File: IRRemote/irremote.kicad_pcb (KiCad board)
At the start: 2 copper layers, 22 parts, among them P1 USB_OTG, P2 TL1838_PINHEADER, P3 DS18B20_PINHEADER_TO92, Q1 Q_NPN_BEC (MMBT2222ALT1G, 145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, Q2 Q_NPN_BEC (MMBT2222ALT1G, 145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, Q3 Q_NPN_BEC (MMBT2222ALT1G, 145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, Q4 Q_NPN_BEC (MMBT2222ALT1G, 145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, U1 ESP-12E, U2 AP1117

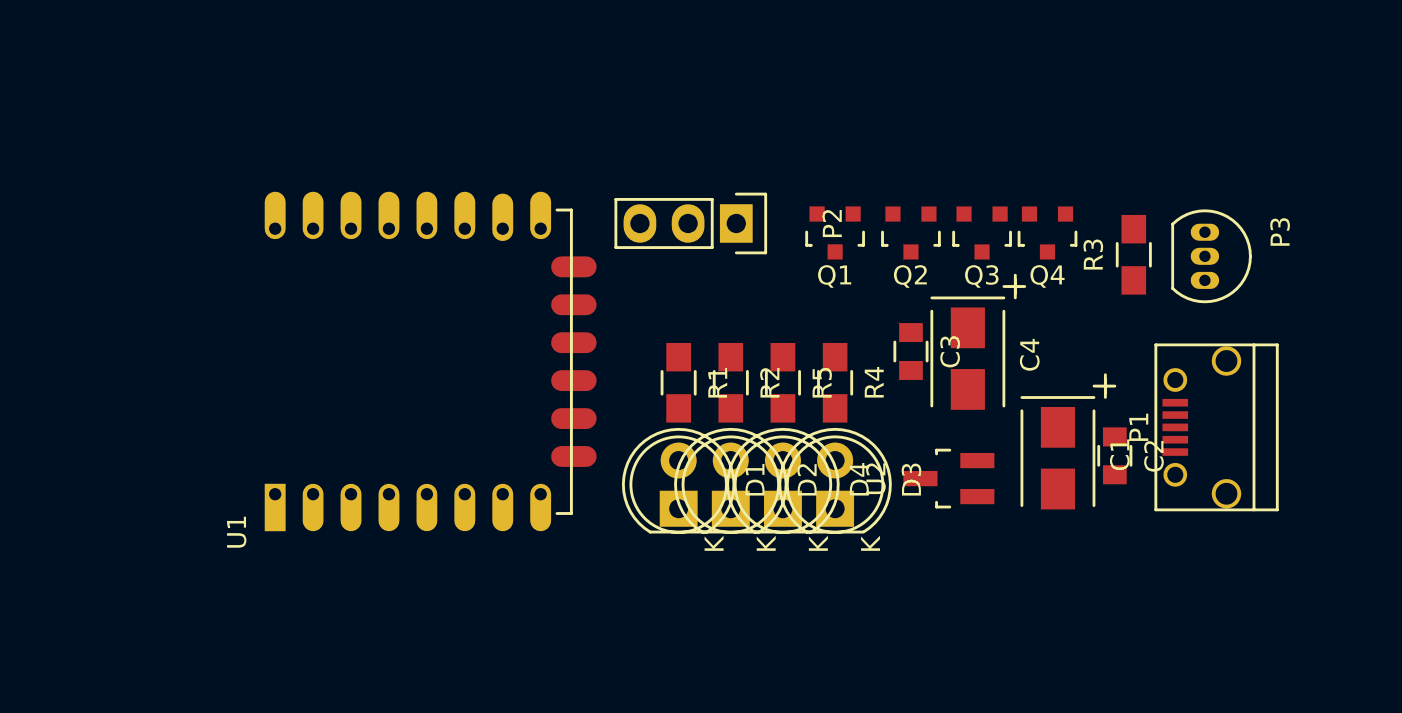
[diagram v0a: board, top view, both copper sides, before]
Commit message: board layout complete
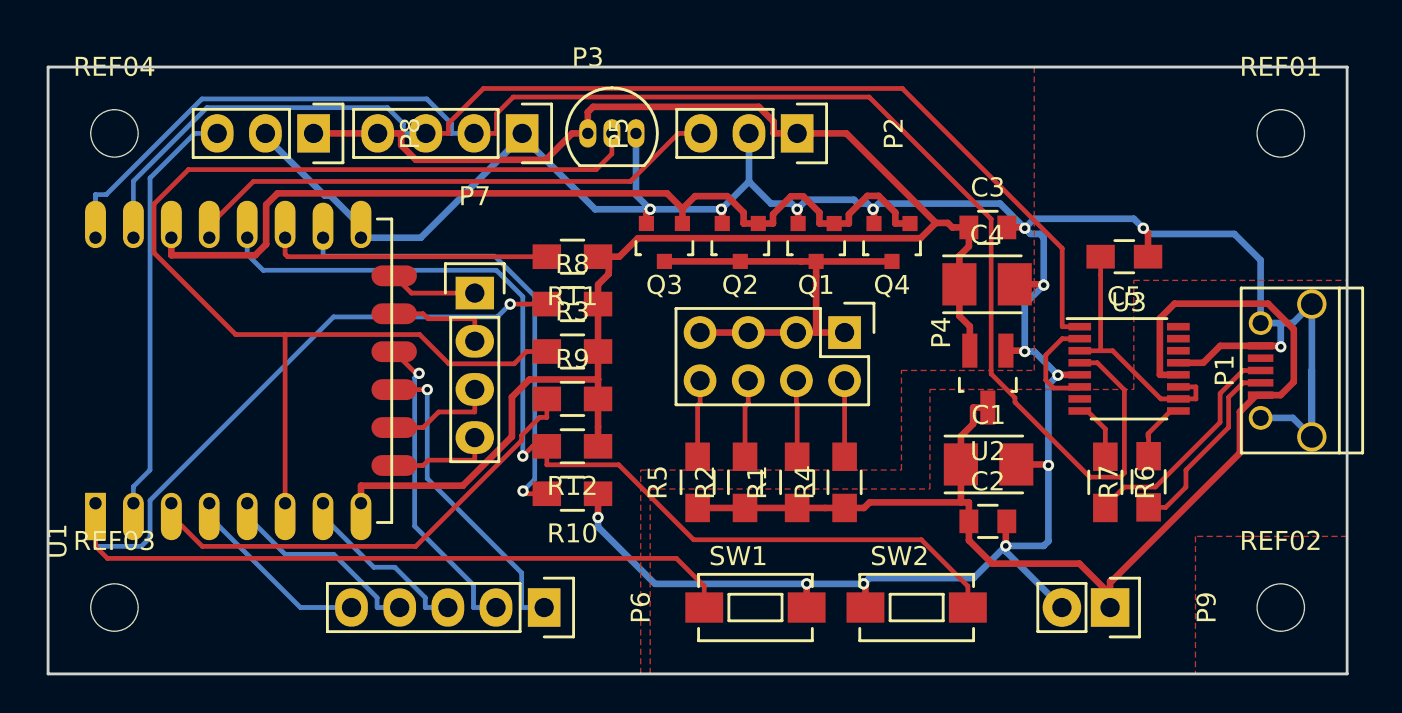
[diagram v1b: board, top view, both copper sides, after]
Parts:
- removed D1, D2, D3, D4: LED, LEDs:LED-5MM
- added C5: C, Capacitors_SMD:C_0805_HandSoldering, F.Cu at (163.2, 61.5)
- added P4: CONN_02X04, Pin_Headers:Pin_Header_Straight_2x04, F.Cu at (148.5, 65.5)
- added P5: CONN_01X04, Pin_Headers:Pin_Header_Straight_1x04, F.Cu at (131.5, 55.0)
- added P6: CONN_01X05, Pin_Headers:Pin_Header_Straight_1x05, F.Cu at (132.7, 80.0)
- added P7: CONN_01X04, Pin_Headers:Pin_Header_Straight_1x04, F.Cu at (129.0, 63.4)
- added P8: TEMP6000, Pin_Headers:Pin_Header_Straight_1x03, F.Cu at (120.5, 55.0)
- added P9: CONN_01X02, Pin_Headers:Pin_Header_Straight_1x02, F.Cu at (162.5, 80.0)
- added R10: 4.7k, Resistors_SMD:R_0805_HandSoldering, F.Cu at (134.2, 74.0)
- added R11: 4.7k, Resistors_SMD:R_0805_HandSoldering, F.Cu at (134.2, 61.5)
- added R12: 4.7k, Resistors_SMD:R_0805_HandSoldering, F.Cu at (134.2, 71.5)
- added R6: 27, Resistors_SMD:R_0805_HandSoldering, F.Cu at (162.2, 73.4)
- added R7: 27, Resistors_SMD:R_0805_HandSoldering, F.Cu at (164.5, 73.4)
- added R8: 4.7k, Resistors_SMD:R_0805_HandSoldering, F.Cu at (134.2, 64.0)
- added R9: 4.7k, Resistors_SMD:R_0805_HandSoldering, F.Cu at (134.2, 69.0)
- added REF01: MountingHole_2-5mm, Mounting_Holes:MountingHole_2-5mm, F.Cu at (171.5, 55.0)
- added REF02: MountingHole_2-5mm, Mounting_Holes:MountingHole_2-5mm, F.Cu at (171.5, 80.0)
- added REF03: MountingHole_2-5mm, Mounting_Holes:MountingHole_2-5mm, F.Cu at (110.0, 80.0)
- added REF04: MountingHole_2-5mm, Mounting_Holes:MountingHole_2-5mm, F.Cu at (110.0, 55.0)
- added SW1: SW_PUSH, Buttons_Switches_SMD:SW_SPST_EVQPE1, F.Cu at (143.8, 80.0)
- added SW2: SW_PUSH, Buttons_Switches_SMD:SW_SPST_EVQPE1, F.Cu at (152.3, 80.0)
- added U3: FT230XS, Housings_SSOP:SSOP-16_3.9x4.9mm_Pitch0.635mm, F.Cu at (163.5, 67.4)
- C1, C4: footprint Capacitors_Tantalum_SMD:TantalC_SizeB_EIA-3528_Wave -> Capacitors_Tantalum_SMD:TantalC_SizeB_EIA-3528_Reflow
- moved P3 33.0 mm to (135.0, 55.0), turned to 0 degrees
- moved R3 30.0 mm to (134.2, 66.5), turned to 0 degrees
- moved Q3 16.8 mm to (139.0, 60.8)
- moved U1 9.49 mm to (109.0, 74.5)
- moved Q2 9.01 mm to (143.0, 60.8)
- moved Q4 8.22 mm to (151.0, 60.8)
- moved R1 8.16 mm to (146.0, 73.4), turned to 90 degrees
- moved C3 7.70 mm to (156.1, 60.0), turned to 0 degrees
- moved C2 7.54 mm to (156.1, 75.5), turned to 0 degrees
- moved R5 6.91 mm to (140.8, 73.4), turned to 90 degrees
- moved P2 5.73 mm to (146.0, 55.0)
- moved U2 5.63 mm to (156.1, 68.0), turned to 180 degrees
- moved P1 5.41 mm to (172.0, 67.5)
- moved R2 5.30 mm to (143.2, 73.4), turned to 90 degrees
- moved R4 5.27 mm to (148.5, 73.4), turned to 90 degrees
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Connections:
- net Net-(D1-Pad1) renamed LED_DR_5
- P1 pad 2: (no net) -> USBDM_1_N
- P1 pad 3: (no net) -> USBDP_1_P
- U1 pad 1: (no net) -> Net-(R8-Pad1)
- U1 pad 10: (no net) -> Net-(P7-Pad3)
- U1 pad 11: (no net) -> Net-(P6-Pad1)
- U1 pad 12: (no net) -> Net-(P6-Pad2)
- U1 pad 13: (no net) -> Net-(P7-Pad2)
- U1 pad 14: (no net) -> Net-(P7-Pad1)
- U1 pad 16: (no net) -> Net-(R10-Pad2)
- U1 pad 17: (no net) -> Net-(R11-Pad2)
- U1 pad 18: (no net) -> Net-(R12-Pad2)
- U1 pad 2: (no net) -> TEMT
- U1 pad 21: (no net) -> TXD_UA_1
- U1 pad 22: (no net) -> RXD_UA_1
- U1 pad 3: (no net) -> Net-(R9-Pad1)
- U1 pad 4: (no net) -> Net-(P6-Pad5)
- U1 pad 5: (no net) -> Net-(P6-Pad4)
- U1 pad 7: (no net) -> Net-(P6-Pad3)
- U1 pad 9: (no net) -> Net-(P7-Pad4)
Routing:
- net GND: track 0.00 -> 163.2 mm, vias 0 -> 15
- net +3V3: track 0.00 -> 93.0 mm
- net RXD_UA_1: track 0.00 -> 81.7 mm
- net Net-(R8-Pad1): track 0.00 -> 68.9 mm, vias 0 -> 1
- net TXD_UA_1: track 0.00 -> 64.3 mm
- net +5V: track 0.00 -> 62.5 mm
- net TEMP_READ: track 0.00 -> 61.2 mm
- net Net-(R12-Pad2): track 0.00 -> 53.2 mm, vias 0 -> 1
- net LED_DR: track 0.00 -> 48.4 mm
- net IR_IN: track 0.00 -> 28.6 mm
- net Net-(R9-Pad1): track 0.00 -> 25.1 mm
- net Net-(R10-Pad2): track 0.00 -> 24.9 mm, vias 0 -> 1
- net LED_DR_5: track 0.00 -> 23.4 mm
- net TEMT: track 0.00 -> 22.0 mm
- net Net-(P6-Pad2): track 0.00 -> 16.7 mm, vias 0 -> 1
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- added copper zone on F.Cu, net +3V3
- added copper zone on F.Cu, net +5V
- added copper zone on B.Cu, net GND
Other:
- board outline added: 68.5 x 32 mm
- net class 3v added: clearance 0.2, trace_width 0.35, via_dia 0.6, via_drill 0.4
- net class 5v added: clearance 0.2, trace_width 0.35, via_dia 0.6, via_drill 0.4
- net class GND added: clearance 0.2, trace_width 0.35, via_dia 0.6, via_drill 0.4
